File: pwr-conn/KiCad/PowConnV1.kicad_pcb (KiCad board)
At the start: 2 copper layers, 17.3 x 21.5 mm, 5 parts, among them P1 8Pin_2x4_inline, P2 PAD, P3 PAD, P4 PAD, P5 PAD

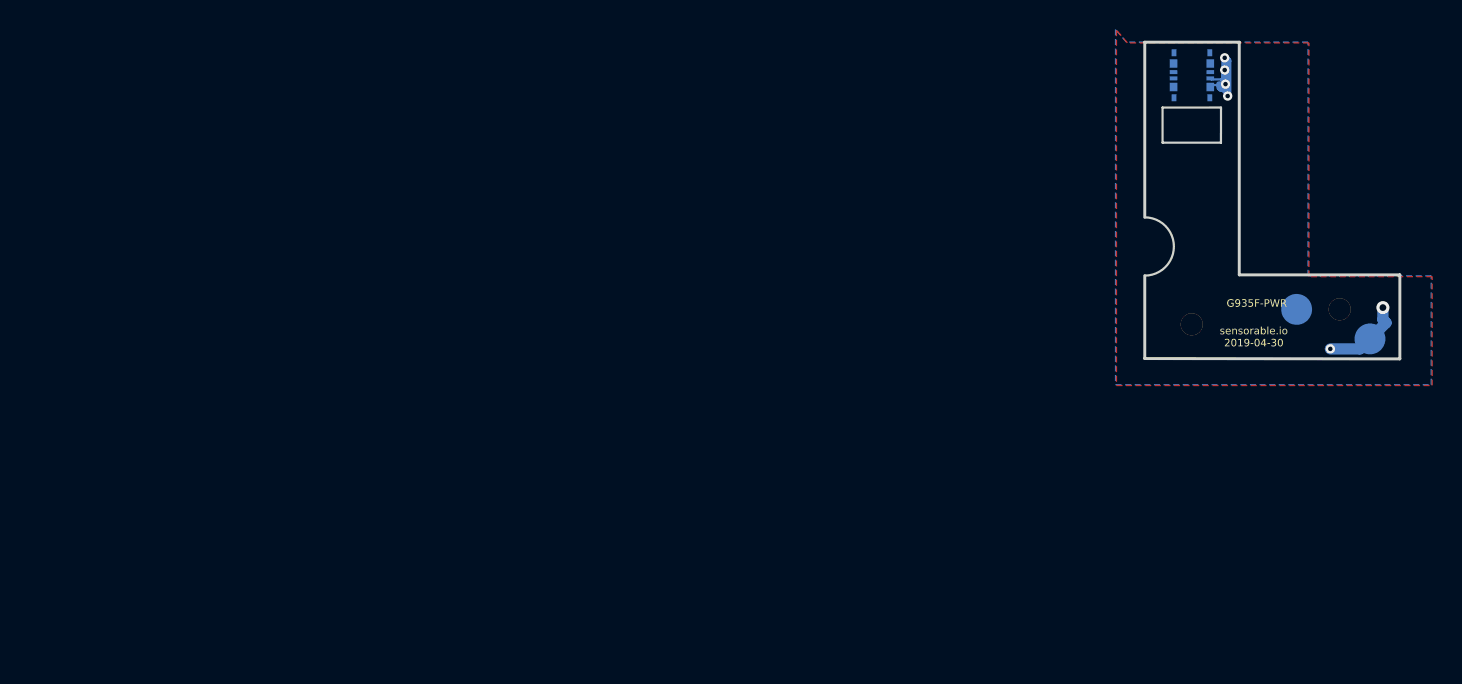
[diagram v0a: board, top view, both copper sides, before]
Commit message: kicad files, ready for assembly
as processed for the mfg+assembly .zip
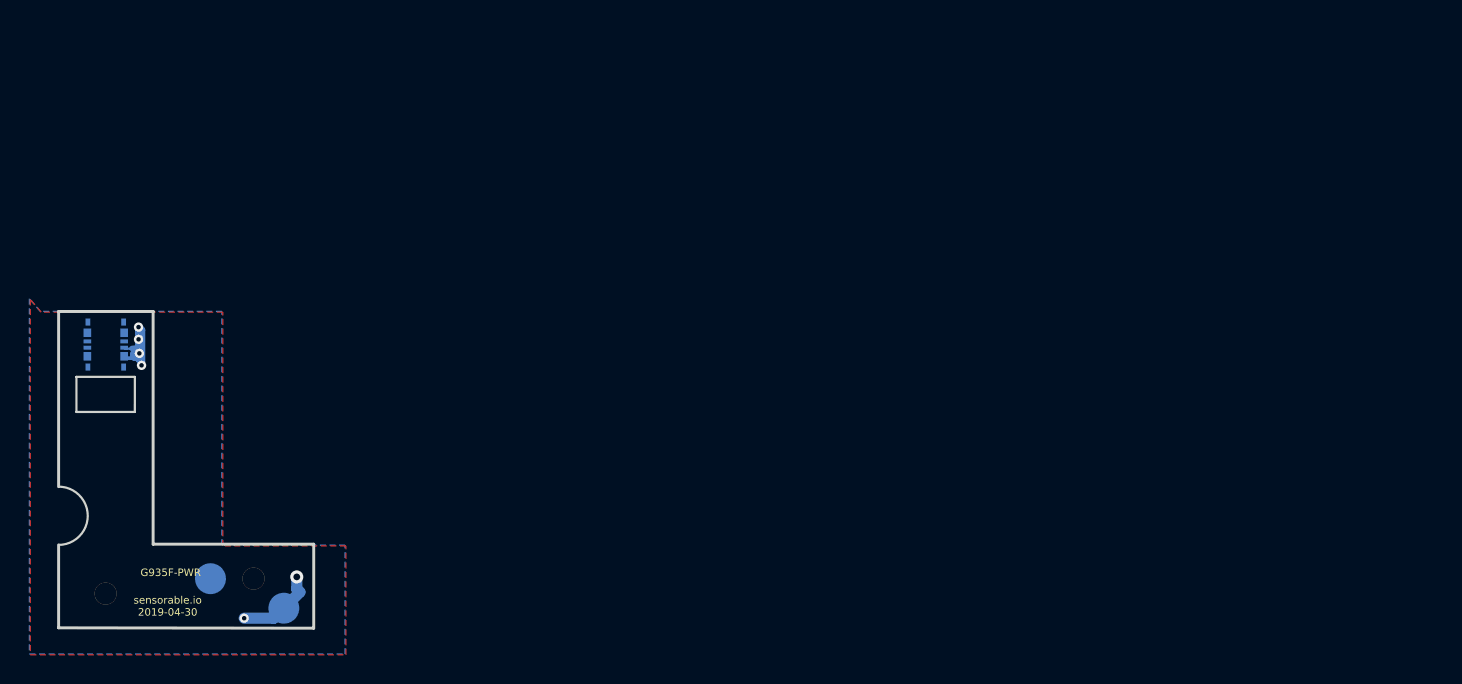
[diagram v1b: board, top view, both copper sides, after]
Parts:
- moved P1 76.1 mm to (40.3, 96.4)
- moved P2 76.1 mm to (40.3, 113.4)
- moved P3 76.1 mm to (50.3, 112.3)
- moved P4 76.1 mm to (52.4, 114.4)
- moved P5 76.1 mm to (47.4, 112.4)
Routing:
- net Dev+: track 20.1 -> 21.0 mm
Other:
- board text added: "Assembly Instructions:"
- board text added: "Copper Layers: 2 Soldermask Layers: 2 Silkscreen Layers: 2 All Layers: Trace Width / Trace Spacing : 6/6 mil Outer Layers: 1 oz copper Inner Layers: .5 oz copper Minimum Via Annular Ring / Drill Diameter: 25mil / 12mil Dielectric: FR-4 Finished board thickness: 1.0mm +- 10%"
- board text added: "Direction of Unreeling"
- board text added: "FILE DESCRIPTIONS:"
- board text added: "Figure 1"
- board text added: "Front Face Orientation"
- board text added: "Orientation 0 degrees"
- board text added: "Orientation 180 degrees"
- board text added: "Orientation 270 degrees"
- board text added: "Orientation 90 degrees"
- board text added: "PCB Manufacturing Requirements:"
- board text added: "Please ask for clarification if any instructions are unclear. Assembly Instructions: 1. The .POS file contains centroid X-Y data and orientation. Orientation is such that 0 degrees indicates placement as if the reel sprocket holes are NORTH of the component. Refer to Figure 1. Do not place any items labeled as DNU. 2. BOM.csv containts BOM, quantities, and part numbers. Please advise before makin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"
- board text added: "Reel"
- board text added: "Round Sprocket Holes"
- board text added: "~~~~~~~~~~~~~~~~~~~~~~~~~~~~~~~~~~~~~~~~~~~~~~~~~~~~~~~~~~~~~~~~~~~~~~~~~~~~~~~~~~~~~~~~~~~~~~~~~~~~~~~~~~~~~~~~~~~~~~~~~~~~~~~~~~~~~~~~~~~~~~~~~~~~~~~~~~~~~~~~~~~~~~ ~~~~~~~~~~~~~~~~~~~~~~~~~~~~~~~~~~~~~~~~~~~~~~~~~~~~~~~~~~~~~~~~~~~~~~~~~~~~~~~~~~~~~~~~~~~~~~~~~~~~~~~~~~~~~~~~~~~~~~~~~~~~~~~~~~~~~~~~~~~~~~~~~~~~~~~~~~~~~~~~~~~~~~ Manufacturing Gerber Files -- Files needed for PCB Manufacturing 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"
